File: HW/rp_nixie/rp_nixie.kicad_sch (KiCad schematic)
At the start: 0 parts

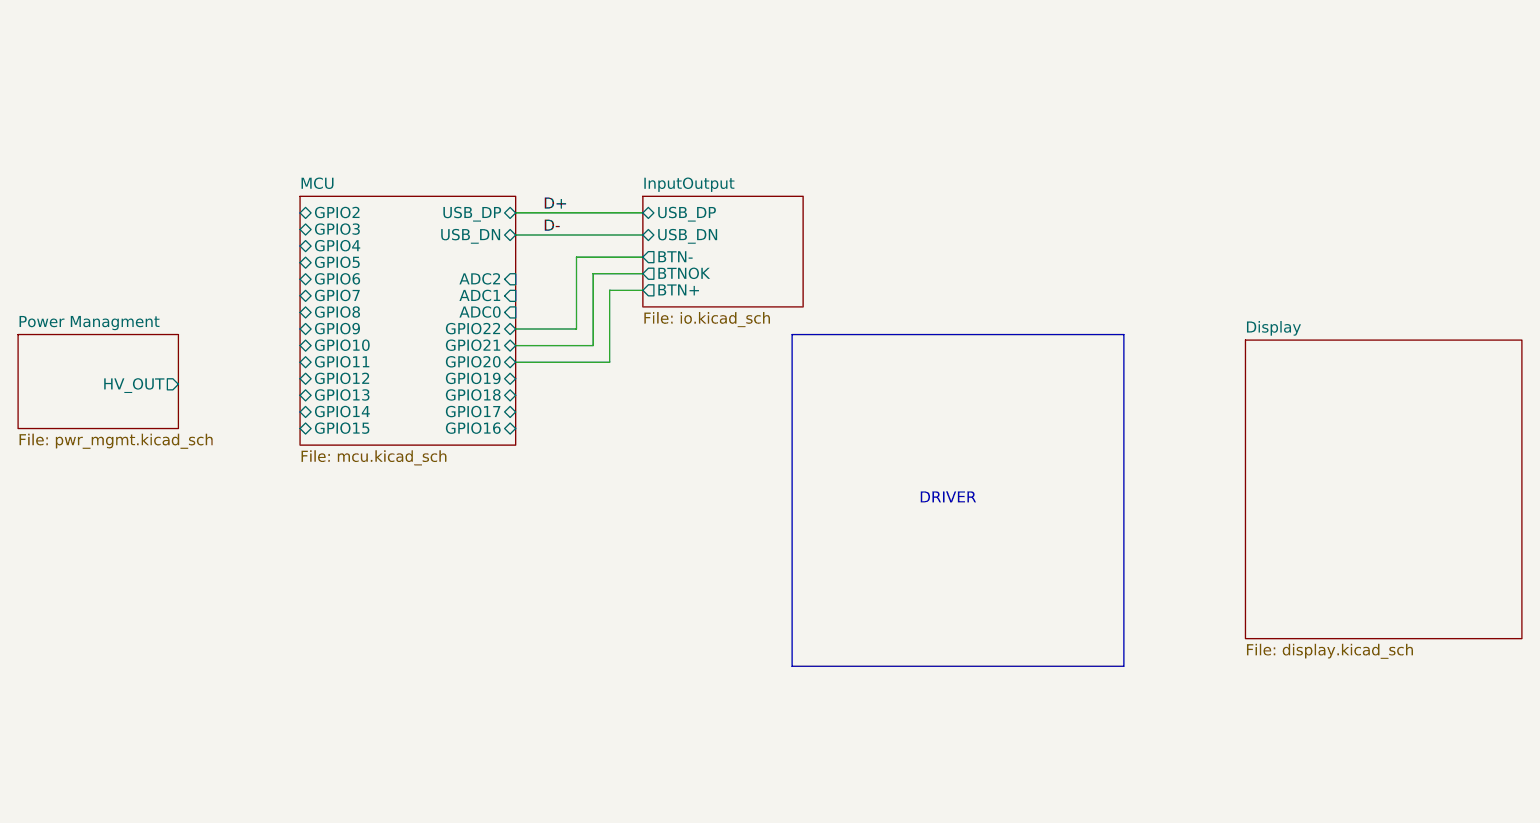
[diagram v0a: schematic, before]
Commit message: some schematic work
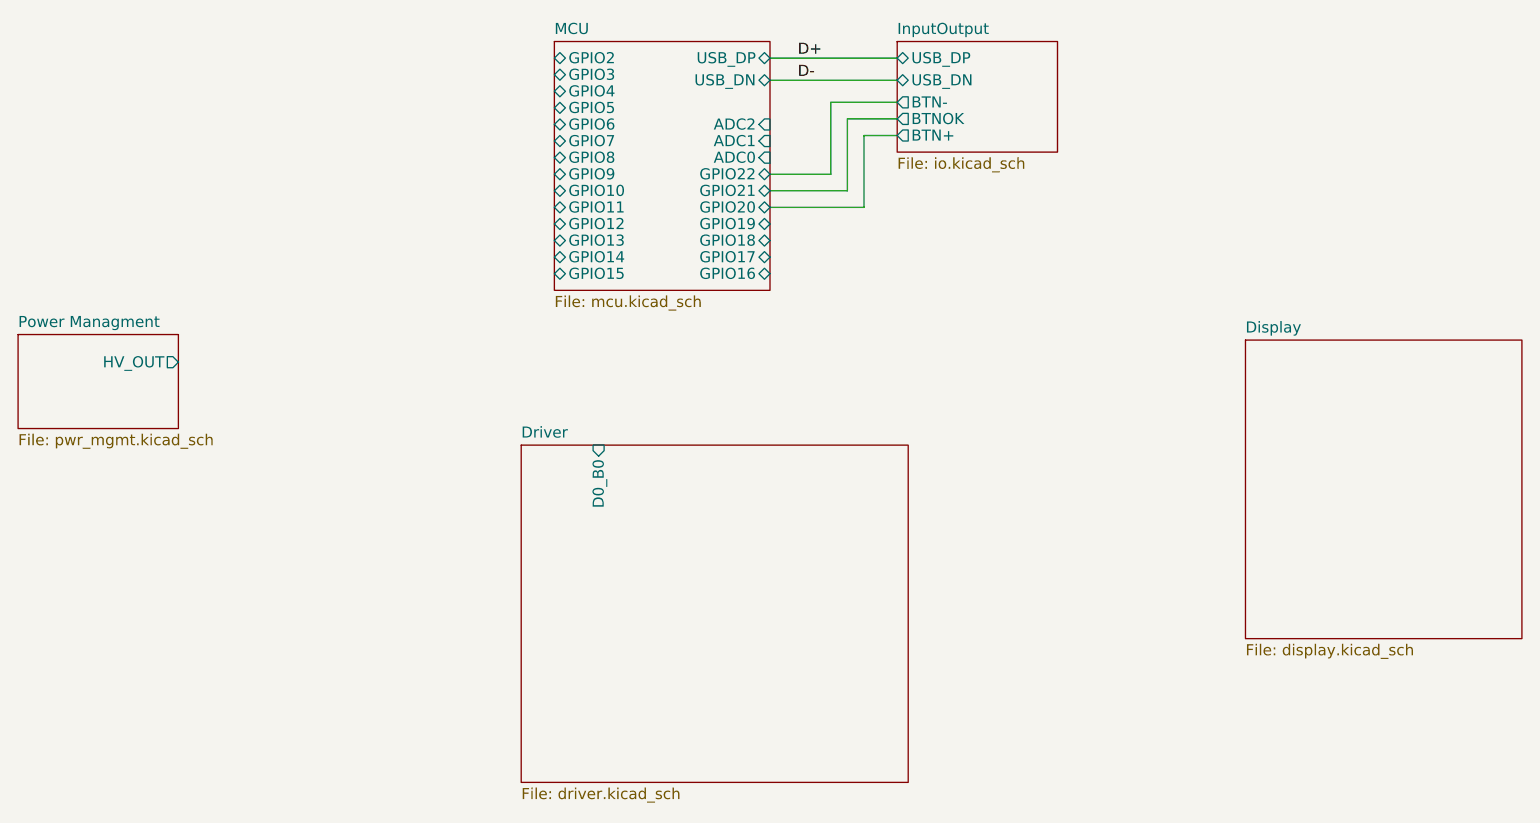
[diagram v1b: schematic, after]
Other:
- added sheet Driver (driver.kicad_sch)
- note removed: "DRIVER"
